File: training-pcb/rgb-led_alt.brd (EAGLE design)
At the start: 30 x 30 mm, 23 parts, among them J1 MICRO-USB, J2 AVR_SPI_PROG2PTH2, K1 SKQGADE010, U1 ATTINY441/841SSU/SSUR, U2 PCA9533

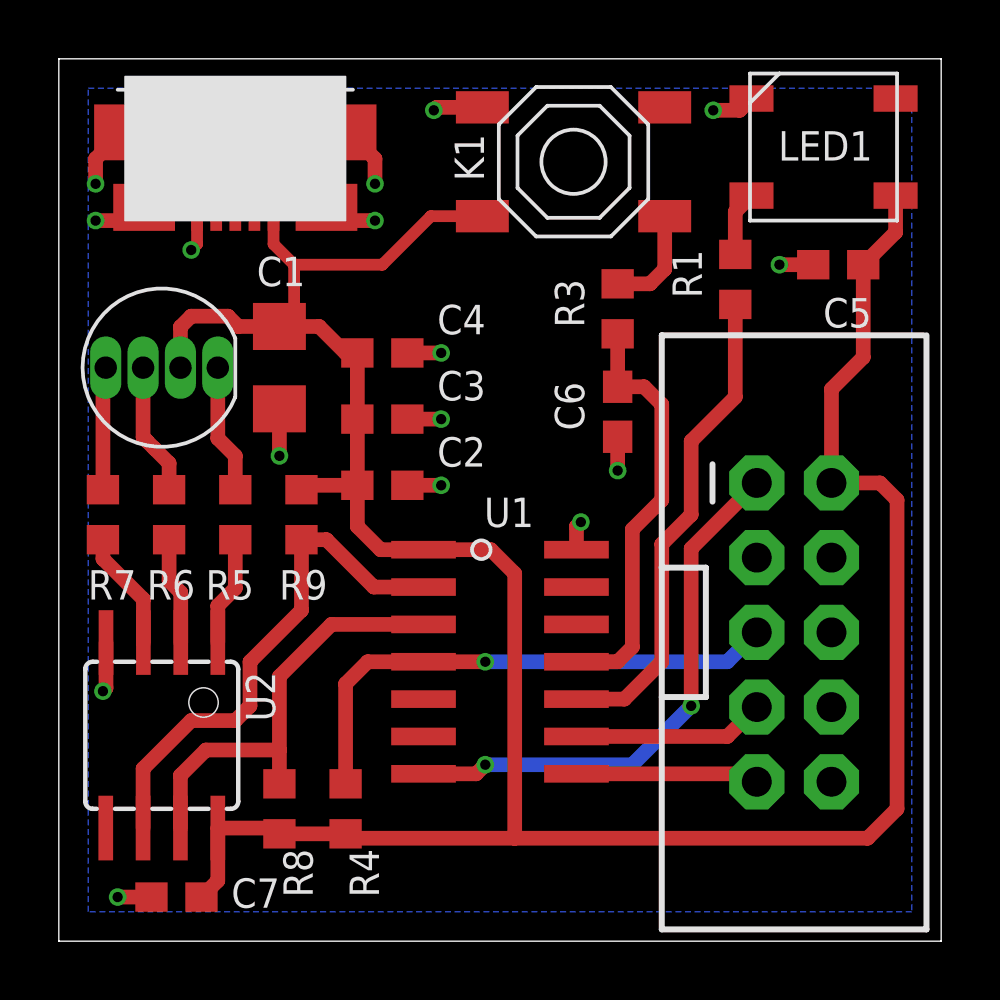
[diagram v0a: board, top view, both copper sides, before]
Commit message: Removed the Series Resistor Instead
Pull-Up was OK
The 0.1uF capacitor should be sufficient to remove switch bounce
All silkscreen has been moved to the top layer
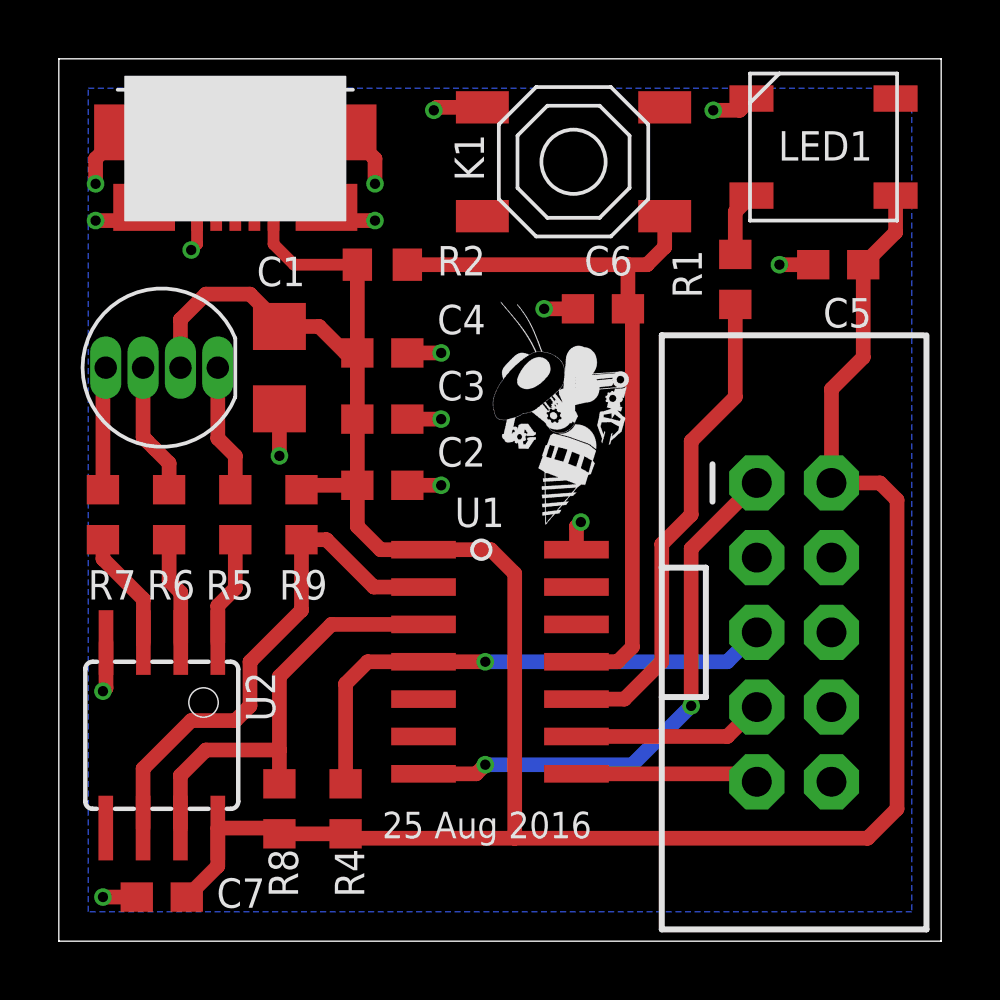
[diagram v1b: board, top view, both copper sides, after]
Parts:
- removed R3: 10k, resistor:R0603
- added R2: 10k, resistor:R0603
- moved U$2 6.63 mm to (16.5, 14.2), flipped to the top
- moved C6 3.54 mm to (18.5, 21.5), turned to 180 degrees
- moved C7 0.50 mm to (3.50, 1.50)
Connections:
- removed net N$3: K1.1, R3.1
- net !BTN: now also K1.1, R2.1; no longer R3.2
- net +5V: now also R2.2; no longer K1.2
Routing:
- net !BTN: track 14.3 -> 25.2 mm
- net N$3: track 3.61 -> 0.00 mm
- net +5V: track 92.4 -> 89.1 mm
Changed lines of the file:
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@@
 <wire x1="30" y1="30" x2="30" y2="0" width="0" layer="20"/>
 <wire x1="30" y1="0" x2="0" y2="0" width="0" layer="20"/>
-<text x="28.5" y="1.5" size="1" layer="22" rot="MR0">25 Aug 2016</text>
+<text x="11" y="3.5" size="0.9" layer="21">25 Aug 2016</text>
 </plain>
 <attributes>
@@
 </element>
 <element name="U1" library="rgb-led" package="SOIC-14" value="ATTINY441/841SSU/SSUR" x="15" y="9.5" smashed="yes" rot="R270">
-<attribute name="NAME" x="14.46" y="14.08" size="1" layer="25"/>
+<attribute name="NAME" x="13.46" y="14.08" size="1" layer="25"/>
 <attribute name="VALUE" x="12.46" y="3.15" size="1.27" layer="27"/>
 </element>
@@
 <attribute name="VALUE" x="3.405" y="13.865" size="1.27" layer="27" rot="R90"/>
 </element>
-<element name="C7" library="rcl" package="C0603" value="0.1uF" x="4" y="1.5" smashed="yes" rot="R180">
-<attribute name="NAME" x="5.865" y="1.135" size="1" layer="25"/>
-<attribute name="VALUE" x="4.635" y="3.405" size="1.27" layer="27" rot="R180"/>
+<element name="C7" library="rcl" package="C0603" value="0.1uF" x="3.5" y="1.5" smashed="yes" rot="R180">
+<attribute name="NAME" x="5.365" y="1.135" size="1" layer="25"/>
+<attribute name="VALUE" x="4.135" y="3.405" size="1.27" layer="27" rot="R180"/>
 </element>
 <element name="R9" library="resistor" package="R0603" value="10k" x="8.25" y="14.5" smashed="yes" rot="R90">
@@
 </element>
 <element name="R8" library="resistor" package="R0603" value="10k" x="7.5" y="4.5" smashed="yes" rot="R270">
-<attribute name="NAME" x="7.635" y="3.135" size="1" layer="25" rot="R270"/>
+<attribute name="NAME" x="7.135" y="3.135" size="1" layer="25" rot="R270"/>
 <attribute name="VALUE" x="5.595" y="5.135" size="1.27" layer="27" rot="R270"/>
 </element>
@@
 <attribute name="VALUE" x="19.405" y="30.183" size="0.889" layer="27" ratio="11" rot="R180"/>
 </element>
-<element name="C6" library="rcl" package="C0603" value="0.1uF" x="19" y="18" smashed="yes" rot="R270">
-<attribute name="NAME" x="17.865" y="17.365" size="1" layer="25" rot="R90"/>
-<attribute name="VALUE" x="17.095" y="18.635" size="1.27" layer="27" rot="R270"/>
-</element>
-<element name="R3" library="resistor" package="R0603" value="10k" x="19" y="21.5" smashed="yes" rot="R270">
-<attribute name="NAME" x="17.865" y="20.865" size="1" layer="25" rot="R90"/>
-<attribute name="VALUE" x="17.095" y="22.135" size="1.27" layer="27" rot="R270"/>
+<element name="R2" library="resistor" package="R0603" value="10k" x="11" y="23" smashed="yes" rot="R180">
+<attribute name="NAME" x="12.865" y="22.635" size="1" layer="25"/>
+<attribute name="VALUE" x="11.635" y="24.905" size="1.27" layer="27" rot="R180"/>
+</element>
+<element name="C6" library="rcl" package="C0603" value="0.1uF" x="18.5" y="21.5" smashed="yes" rot="R180">
+<attribute name="NAME" x="17.865" y="22.635" size="1" layer="25"/>
+<attribute name="VALUE" x="19.135" y="23.405" size="1.27" layer="27" rot="R180"/>
 </element>
 <element name="R4" library="resistor" package="R0603" value="10k" x="9.75" y="4.5" smashed="yes" rot="R270">
-<attribute name="NAME" x="9.885" y="3.135" size="1" layer="25" rot="R270"/>
+<attribute name="NAME" x="9.385" y="3.135" size="1" layer="25" rot="R270"/>
 <attribute name="VALUE" x="7.845" y="5.135" size="1.27" layer="27" rot="R270"/>
 </element>
-<element name="U$2" library="RoboJackets-Aesthetics" package="ROBOBUZZ_0.4X" value="" x="15.22" y="20.66" smashed="yes" rot="MR0"/>
+<element name="U$2" library="RoboJackets-Aesthetics" package="ROBOBUZZ_0.4X" value="" x="16.53" y="14.16" smashed="yes"/>
 </elements>
 <signals>
@@
 <via x="10.75" y="25.75" extent="1-16" drill="0.35"/>
 <via x="24.5" y="23" extent="1-16" drill="0.35"/>
-<via x="2" y="1.5" extent="1-16" drill="0.35"/>
+<via x="1.5" y="1.5" extent="1-16" drill="0.35"/>
 <via x="1.25" y="24.5" extent="1-16" drill="0.35"/>
 <via x="1.25" y="25.75" extent="1-16" drill="0.35"/>
 <via x="1.5" y="8.5" extent="1-16" drill="0.35"/>
-<via x="19" y="16" extent="1-16" drill="0.35"/>
+<via x="16.5" y="21.5" extent="1-16" drill="0.35"/>
 <wire x1="17.6" y1="13.31" x2="17.6" y2="14.1" width="0.5" layer="1"/>
 <wire x1="17.6" y1="14.1" x2="17.75" y2="14.25" width="0.5" layer="1"/>
-<wire x1="3.15" y1="1.5" x2="2" y2="1.5" width="0.5" layer="1"/>
+<wire x1="2.65" y1="1.5" x2="1.5" y2="1.5" width="0.5" layer="1"/>
 <wire x1="1.605" y1="10.154" x2="1.605" y2="8.605" width="0.5" layer="1"/>
 <wire x1="1.605" y1="8.605" x2="1.5" y2="8.5" width="0.5" layer="1"/>
@@
 <wire x1="22.25" y1="28.25" x2="23.15" y2="28.25" width="0.5" layer="1"/>
 <wire x1="23.15" y1="28.25" x2="23.55" y2="28.65" width="0.5" layer="1"/>
-<wire x1="19" y1="17.15" x2="19" y2="16" width="0.5" layer="1"/>
+<wire x1="17.65" y1="21.5" x2="16.5" y2="21.5" width="0.5" layer="1"/>
 <wire x1="14.4" y1="28.35" x2="12.85" y2="28.35" width="0.5" layer="1"/>
 <wire x1="12.85" y1="28.35" x2="12.75" y2="28.25" width="0.5" layer="1"/>
@@
 <contactref element="C5" pad="1"/>
 <contactref element="J1" pad="1"/>
+<contactref element="R2" pad="2"/>
 <contactref element="U2" pad="8"/>
 <contactref element="C7" pad="1"/>
@@
 <wire x1="26.27" y1="18.77" x2="27.35" y2="19.85" width="0.5" layer="1"/>
 <wire x1="27.35" y1="23" x2="27.35" y2="19.85" width="0.5" layer="1"/>
-<wire x1="5.405" y1="3.846" x2="5.405" y2="2.055" width="0.5" layer="1"/>
-<wire x1="5.405" y1="2.055" x2="4.85" y2="1.5" width="0.5" layer="1"/>
+<wire x1="5.405" y1="3.846" x2="5.405" y2="2.555" width="0.5" layer="1"/>
+<wire x1="5.405" y1="2.555" x2="4.35" y2="1.5" width="0.5" layer="1"/>
 <wire x1="5.405" y1="3.846" x2="7.304" y2="3.846" width="0.5" layer="1"/>
 <wire x1="7.304" y1="3.846" x2="7.5" y2="3.65" width="0.5" layer="1"/>
@@
 <wire x1="10.15" y1="15.5" x2="8.4" y2="15.5" width="0.5" layer="1"/>
 <wire x1="8.4" y1="15.5" x2="8.25" y2="15.35" width="0.5" layer="1"/>
+<wire x1="10.15" y1="23" x2="10.15" y2="20" width="0.5" layer="1"/>
 <wire x1="28.45" y1="25.35" x2="28.45" y2="24.1" width="0.5" layer="1"/>
 <wire x1="28.45" y1="24.1" x2="27.35" y2="23" width="0.5" layer="1"/>
@@
 <wire x1="12.4" y1="13.31" x2="10.94" y2="13.31" width="0.5" layer="1"/>
 <wire x1="10.94" y1="13.31" x2="10.15" y2="14.1" width="0.5" layer="1"/>
+<wire x1="4.135" y1="19.5" x2="4.135" y2="21.135" width="0.5" layer="1"/>
 <wire x1="7.5" y1="20.9" x2="8.85" y2="20.9" width="0.5" layer="1"/>
 <wire x1="8.85" y1="20.9" x2="9.75" y2="20" width="0.5" layer="1"/>
 <wire x1="10.15" y1="20" x2="9.75" y2="20" width="0.5" layer="1"/>
 <wire x1="7.5" y1="20.9" x2="7.5" y2="21" width="0.5" layer="1"/>
+<wire x1="7.5" y1="21" x2="6.5" y2="22" width="0.5" layer="1"/>
+<wire x1="6.5" y1="22" x2="5" y2="22" width="0.5" layer="1"/>
+<wire x1="5" y1="22" x2="4.135" y2="21.135" width="0.5" layer="1"/>
 <wire x1="7.3" y1="24.825" x2="7.3" y2="23.7" width="0.4" layer="1"/>
 <wire x1="7.3" y1="23.7" x2="8" y2="23" width="0.4" layer="1"/>
-<contactref element="K1" pad="2"/>
-<wire x1="14.4" y1="24.65" x2="12.65" y2="24.65" width="0.4" layer="1"/>
-<wire x1="12.65" y1="24.65" x2="11" y2="23" width="0.4" layer="1"/>
-<wire x1="8" y1="23" x2="11" y2="23" width="0.4" layer="1"/>
-<wire x1="8" y1="23" x2="8" y2="21.4" width="0.4" layer="1"/>
-<wire x1="8" y1="21.4" x2="7.5" y2="20.9" width="0.4" layer="1"/>
-<wire x1="7.5" y1="20.9" x2="6.1" y2="20.9" width="0.5" layer="1"/>
-<wire x1="6.1" y1="20.9" x2="5.75" y2="21.25" width="0.5" layer="1"/>
-<wire x1="4.135" y1="19.5" x2="4.135" y2="20.885" width="0.5" layer="1"/>
-<wire x1="4.135" y1="20.885" x2="4.5" y2="21.25" width="0.5" layer="1"/>
-<wire x1="4.5" y1="21.25" x2="5.75" y2="21.25" width="0.5" layer="1"/>
+<wire x1="8" y1="23" x2="10.15" y2="23" width="0.4" layer="1"/>
 </signal>
 <signal name="MOSI">
@@
 <signal name="!BTN">
 <contactref element="C6" pad="1"/>
-<contactref element="R3" pad="2"/>
 <contactref element="U1" pad="11"/>
 <wire x1="17.6" y1="9.5" x2="19" y2="9.5" width="0.5" layer="1"/>
 <wire x1="19" y1="9.5" x2="19.5" y2="10" width="0.5" layer="1"/>
-<wire x1="20.5" y1="18.25" x2="19.9" y2="18.85" width="0.5" layer="1"/>
-<wire x1="19" y1="18.85" x2="19.9" y2="18.85" width="0.5" layer="1"/>
-<wire x1="19.5" y1="10" x2="19.5" y2="14" width="0.5" layer="1"/>
-<wire x1="19.5" y1="14" x2="20.5" y2="15" width="0.5" layer="1"/>
-<wire x1="20.5" y1="15" x2="20.5" y2="18.25" width="0.5" layer="1"/>
-<wire x1="19" y1="20.65" x2="19" y2="18.85" width="0.5" layer="1"/>
-</signal>
-<signal name="N$3">
 <contactref element="K1" pad="1"/>
-<contactref element="R3" pad="1"/>
-<wire x1="19" y1="22.35" x2="20.1" y2="22.35" width="0.5" layer="1"/>
-<wire x1="20.1" y1="22.35" x2="20.6" y2="22.85" width="0.5" layer="1"/>
-<wire x1="20.6" y1="24.65" x2="20.6" y2="22.85" width="0.5" layer="1"/>
+<wire x1="20" y1="23" x2="20.6" y2="23.6" width="0.5" layer="1"/>
+<wire x1="20.6" y1="24.65" x2="20.6" y2="23.6" width="0.5" layer="1"/>
+<contactref element="R2" pad="1"/>
+<wire x1="11.85" y1="23" x2="19.35" y2="23" width="0.5" layer="1"/>
+<wire x1="19.35" y1="23" x2="20" y2="23" width="0.5" layer="1"/>
+<wire x1="19.5" y1="10" x2="19.5" y2="21.35" width="0.5" layer="1"/>
+<wire x1="19.5" y1="21.35" x2="19.35" y2="21.5" width="0.5" layer="1"/>
+<wire x1="19.35" y1="21.5" x2="19.35" y2="23" width="0.5" layer="1"/>
 </signal>
 <signal name="N$4">

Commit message: Optimized a Few Traces
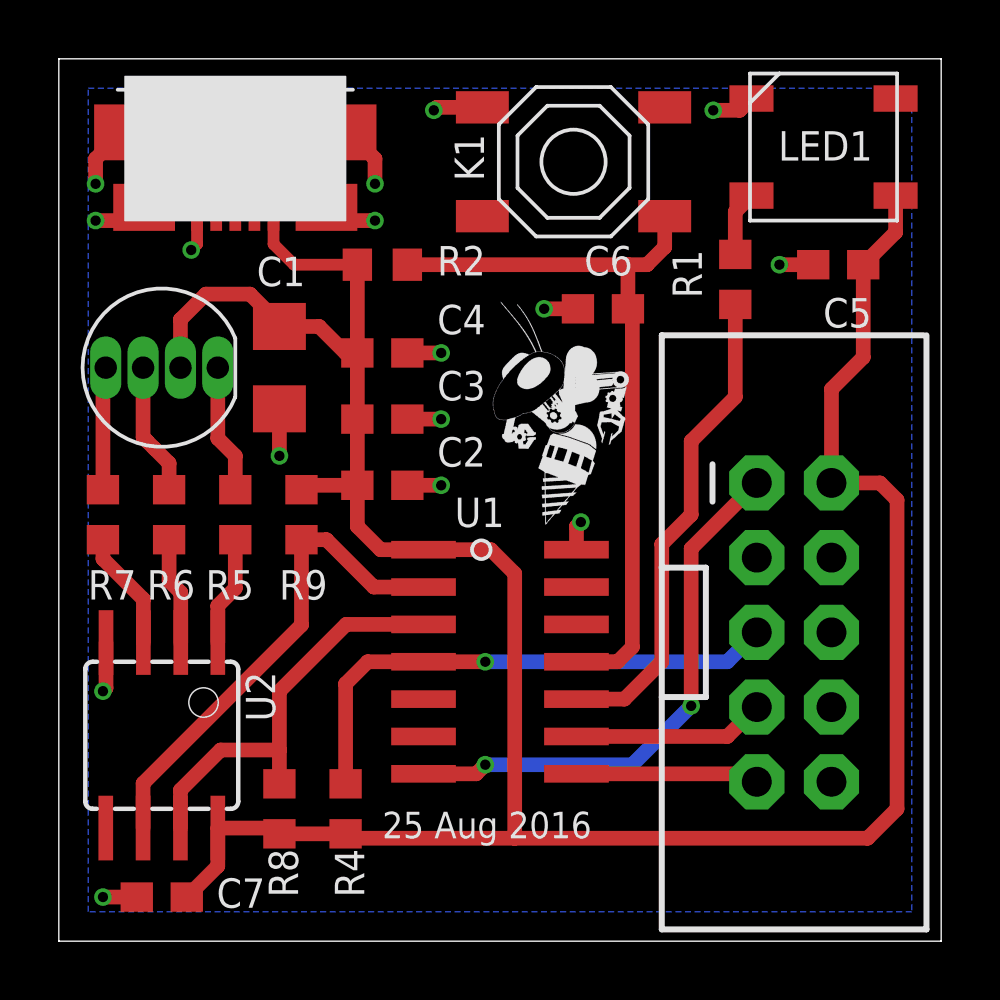
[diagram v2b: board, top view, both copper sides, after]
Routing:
- net SCL: track 17.7 -> 16.9 mm
- net SDA: track 14.8 -> 14.2 mm
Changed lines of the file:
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@@
 <contactref element="U2" pad="6"/>
 <contactref element="R9" pad="1"/>
-<wire x1="2.865" y1="3.846" x2="2.865" y2="5.865" width="0.5" layer="1"/>
-<wire x1="2.865" y1="5.865" x2="4.5" y2="7.5" width="0.5" layer="1"/>
-<wire x1="4.5" y1="7.5" x2="6" y2="7.5" width="0.5" layer="1"/>
-<wire x1="6" y1="7.5" x2="6.5" y2="8" width="0.5" layer="1"/>
-<wire x1="6.5" y1="8" x2="6.5" y2="9.5" width="0.5" layer="1"/>
-<wire x1="6.5" y1="9.5" x2="8.25" y2="11.25" width="0.5" layer="1"/>
-<wire x1="8.25" y1="13.65" x2="8.25" y2="11.25" width="0.5" layer="1"/>
+<wire x1="2.865" y1="3.846" x2="2.865" y2="5.365" width="0.5" layer="1"/>
+<wire x1="2.865" y1="5.365" x2="8.25" y2="10.75" width="0.5" layer="1"/>
+<wire x1="8.25" y1="13.65" x2="8.25" y2="10.75" width="0.5" layer="1"/>
 <wire x1="12.4" y1="12.04" x2="10.71" y2="12.04" width="0.5" layer="1"/>
 <wire x1="10.71" y1="12.04" x2="9.1" y2="13.65" width="0.5" layer="1"/>
@@
 <contactref element="R8" pad="1"/>
 <wire x1="7.5" y1="5.35" x2="7.5" y2="6.5" width="0.5" layer="1"/>
-<wire x1="7.5" y1="6.5" x2="7.5" y2="9" width="0.5" layer="1"/>
-<wire x1="7.5" y1="9" x2="9.27" y2="10.77" width="0.5" layer="1"/>
-<wire x1="12.4" y1="10.77" x2="9.27" y2="10.77" width="0.5" layer="1"/>
-<wire x1="4.135" y1="3.846" x2="4.135" y2="5.635" width="0.5" layer="1"/>
-<wire x1="4.135" y1="5.635" x2="5" y2="6.5" width="0.5" layer="1"/>
-<wire x1="5" y1="6.5" x2="7.5" y2="6.5" width="0.5" layer="1"/>
+<wire x1="7.5" y1="6.5" x2="7.5" y2="8.5" width="0.5" layer="1"/>
+<wire x1="7.5" y1="8.5" x2="9.77" y2="10.77" width="0.5" layer="1"/>
+<wire x1="12.4" y1="10.77" x2="9.77" y2="10.77" width="0.5" layer="1"/>
+<wire x1="4.135" y1="3.846" x2="4.135" y2="5.135" width="0.5" layer="1"/>
+<wire x1="4.135" y1="5.135" x2="5.5" y2="6.5" width="0.5" layer="1"/>
+<wire x1="5.5" y1="6.5" x2="7.5" y2="6.5" width="0.5" layer="1"/>
 </signal>
 <signal name="N$6">
